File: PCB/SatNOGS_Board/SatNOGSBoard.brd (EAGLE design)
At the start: 59.4 x 68.6 mm, 25 parts, among them IC1 MEGA8-AI, IC2 78L05F, J3 4, Q1 16MHz

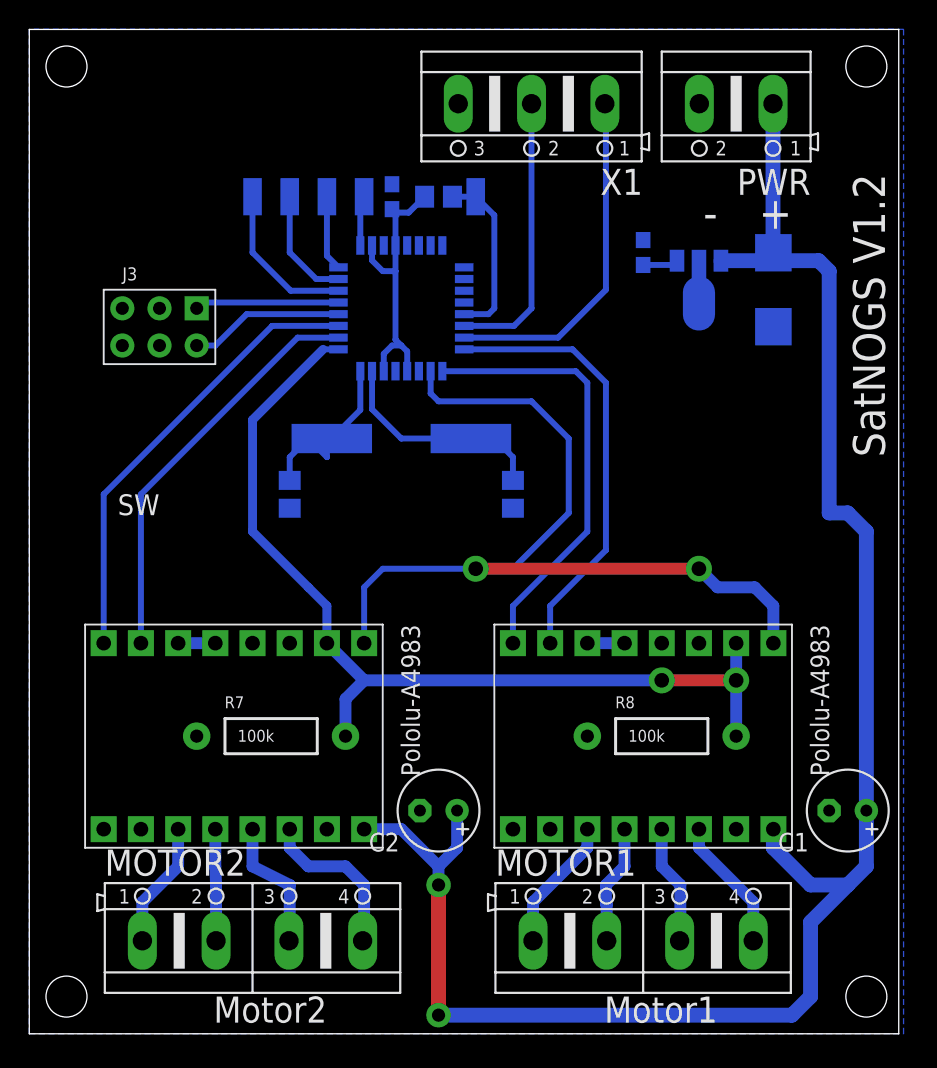
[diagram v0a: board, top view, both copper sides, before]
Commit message: board routing
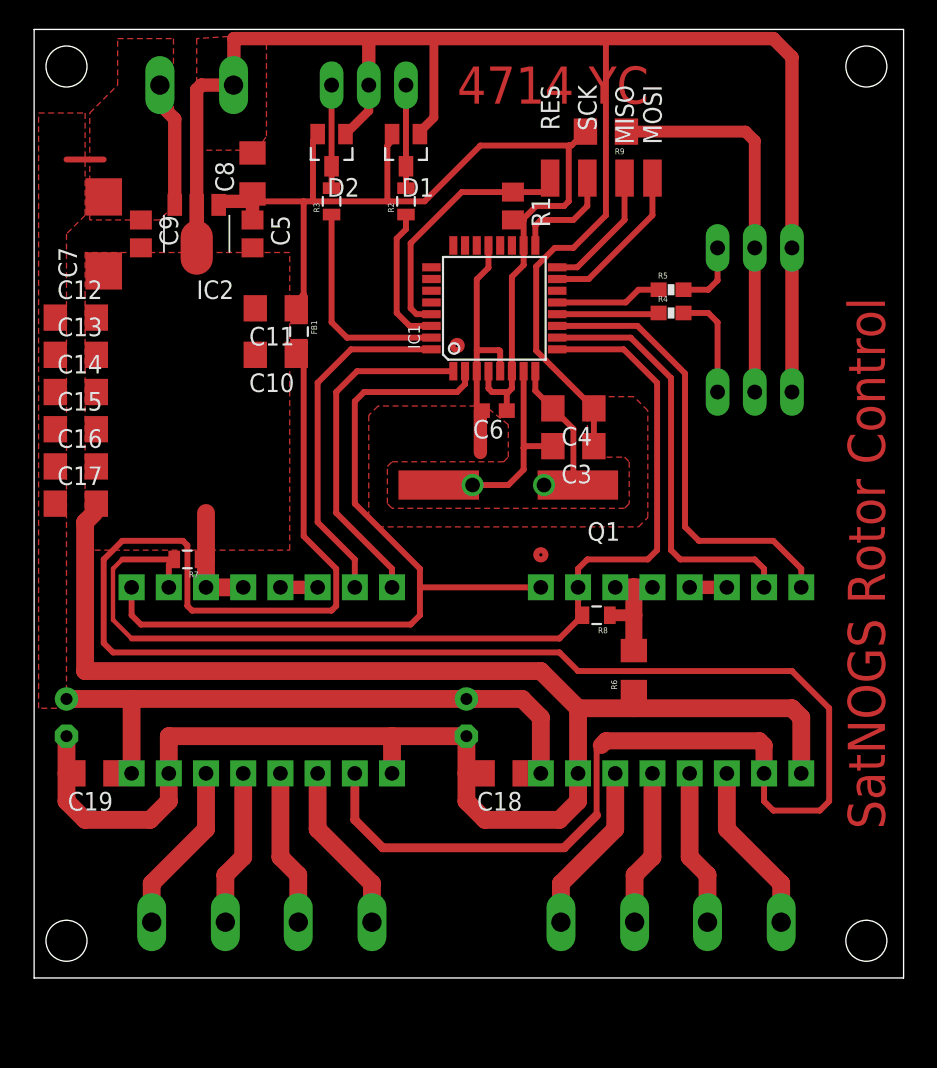
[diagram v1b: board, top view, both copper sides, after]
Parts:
- removed J3: 4, Connector:2X3P-2.54-65/35MIL
- removed PAD1, PAD2, PAD3, PAD4, PAD5: (no value), wirepad:SMD1,27-2,54
- removed X1: (no value), con-ptr500:AK500/3
- added C10, C11, C12, C13, C14, C15, C16, C17, C18, C19, C8: 680n, rcl:C1206
- added C9: 100n, rcl:C0805
- added D1, D2: BAV99, diode:SOT23
- added FB1: 10R@100MHz, SparkFun-Resistors:0805
- added JP1, JP2, JP3: (no value), pinhead:1X03
- added MISO, MOSI, RES, SCK: (no value), wirepad:SMD1,27-2,54
- added R2: 1k, SparkFun-Resistors:0805
- added R3: 475R, SparkFun-Resistors:0805
- added R4, R5: (no value), SparkFun-Resistors:0603-RES
- added R6, R9: 0R, SparkFun-Resistors:1206
- C3, C4: device rcl:C0805 -> rcl:C1206
- C5: device rcl:C0603 -> rcl:C0805
- R1: value 10k -> 4k7
- R7, R8: device SparkFun-Resistors:AXIAL-0.4 -> SparkFun-Resistors:0805
- moved C1 53.7 mm to (2.54, 21.6), flipped to the bottom, turned to 270 degrees
- moved C7 45.9 mm to (5.08, 54.6), flipped to the top
- moved PWR 36.9 mm to (11.4, 64.8), flipped to the bottom
- moved IC2 34.5 mm to (11.4, 54.6), flipped to the top
- moved DRIVER2 30.1 mm to (43.8, 24.1), flipped to the bottom
- moved MOTOR2 28.6 mm to (43.8, 7.62), flipped to the bottom
- moved C5 26.7 mm to (15.2, 54.6), flipped to the top, turned to 270 degrees
- moved DRIVER1 26.3 mm to (15.9, 24.1), flipped to the bottom
- moved MOTOR1 26.1 mm to (15.9, 7.62), flipped to the bottom
- moved C4 20.2 mm to (37.1, 42.7), flipped to the top, turned to 180 degrees
- moved C6 16.2 mm to (31.8, 42.5), flipped to the top, turned to 180 degrees
- moved R7 13.4 mm to (10.8, 32.4), turned to 180 degrees
- moved R8 9.38 mm to (38.7, 28.6), turned to 180 degrees
- moved Q1 7.96 mm to (32.7, 37.5), flipped to the top
- moved C2 6.63 mm to (29.8, 21.6), flipped to the bottom, turned to 270 degrees
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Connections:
- net N$4 renamed XTAL1
- net N$6 renamed XTAL2
- removed net VMOTOR: C1.+, C2.+, C7.+, DRIVER1.16, DRIVER2.16, IC2.3, PWR.1
- new net +12V: C1.+, C12.1, C13.1, C14.1, C15.1, C16.1, C17.1, C18.1, C19.1, C2.+, C7.+, C9.1, DRIVER1.16, DRIVER2.16, IC2.3, PWR.1
- new net +5VM: C10.1, DRIVER1.10, DRIVER2.10, FB1.2
- new net N$12: IC1.12, R4.1
- new net N$13: DRIVER2.3, DRIVER2.4, R6.2, R8.1
- new net N$14: JP2.2, JP3.2, R9.1
- new net N$4: D2.3, JP1.3, R3.2
- new net N$6: IC1.30, R2.1
- net +5V: now also C11.1, C8.1, D1.2, D2.2, FB1.1, R9.2; no longer DRIVER1.10, DRIVER2.10, IC1.20, J3.3, J3.4
- net GND: now also C10.2, C11.2, C12.2, C13.2, C14.2, C15.2, C16.2, C17.2, C18.2, C19.2, C8.2, C9.2, D1.1, D2.1, JP1.2, JP2.3, JP3.3, R6.1, R7.1; no longer DRIVER2.3, DRIVER2.4, J3.2, J3.5, R7.P$1, R8.P$1, X1.3
- net MS1: now also R7.2, R8.2; no longer R7.P$2, R8.P$2
- net N$10: now also MISO.1; no longer PAD2.1
- net N$11: now also SCK.1; no longer PAD1.1
- net N$3: now also D1.3, JP1.1, R2.2; no longer IC1.31, X1.1
- net N$5: now also RES.1; no longer PAD5.1
- net N$7: now also IC1.31, R3.1; no longer IC1.30, X1.2
- net N$8: now also IC1.13, R5.1; no longer IC1.14, PAD4.1
- net N$9: now also MOSI.1; no longer PAD3.1
- net SW1: now also JP2.1, R5.2; no longer IC1.13, J3.1
- net SW2: now also JP3.1, R4.2; no longer IC1.12, J3.6
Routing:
- net GND: track 0.00 -> 278.9 mm
- net +5VM: track 0.00 -> 150.3 mm
- net VMOTOR: track 128.5 -> 0.00 mm, vias 2 -> 0
- net +12V: track 0.00 -> 55.2 mm
- net +5V: track 21.9 -> 71.2 mm
- net N$14: track 0.00 -> 26.2 mm
- net N$3: track 23.8 -> 7.04 mm
- net N$6: track 0.00 -> 9.72 mm
- net N$13: track 0.00 -> 8.50 mm
- net N$4: track 0.00 -> 7.04 mm
- net MS1: track 64.9 -> 71.9 mm, vias 2 -> 0
- net N$12: track 0.00 -> 6.96 mm
- net DIR-1: track 30.1 -> 23.5 mm
- net STEP-1: track 30.0 -> 23.7 mm
- net N$5: track 12.0 -> 17.8 mm
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- added copper zone on layer 1, net +12V
- added copper zone on layer 1, net GND
- removed copper zone on layer 16, net GND
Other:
- board size 59.4 x 68.6 mm -> 59.4 x 64.8 mm
- board text added: "4714 YC"
- board text added: "SatNOGS Rotor Control"
- board text removed: "+"
- board text removed: "-"
- board text removed: "Motor1"
- board text removed: "Motor2"
- board text removed: "SW"
- board text removed: "SatNOGS V1.2"
